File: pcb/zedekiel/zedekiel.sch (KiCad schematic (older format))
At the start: 150 parts, among them K1 KEYSW, K10 KEYSW, K11 KEYSW, K12 KEYSW, K13 KEYSW, K14 KEYSW, K15 KEYSW, K16 KEYSW, K17 KEYSW, K18 KEYSW, K19 KEYSW, K2 KEYSW, K20 KEYSW, K21 KEYSW, K22 KEYSW, K23 KEYSW, K24 KEYSW, K25 KEYSW, K26 KEYSW, K27 KEYSW, K28 KEYSW, K29 KEYSW, K3 KEYSW, K30 KEYSW, K31 KEYSW, K32 KEYSW, K33 KEYSW, K34 KEYSW, K35 KEYSW, K36 KEYSW, K37 KEYSW, K38 KEYSW, K39 KEYSW, K4 KEYSW, K40 KEYSW, K41 KEYSW, K42 KEYSW, K43 KEYSW, K44 KEYSW, K45 KEYSW, K46 KEYSW, K47 KEYSW, K48 KEYSW, K49 KEYSW, K5 KEYSW, K50 KEYSW, K51 KEYSW, K52 KEYSW, K53 KEYSW, K54 KEYSW, K55 KEYSW, K56 KEYSW, K57 KEYSW, K58 KEYSW, K59 KEYSW, K6 KEYSW, K60 KEYSW, K61 KEYSW, K62 KEYSW, K63 KEYSW, K64 KEYSW, K65 KEYSW, K66 KEYSW, K7 KEYSW, K8 KEYSW, K9 KEYSW, SW1 SW_PUSH, U1 ATmega16U4-AU_(modified), X1 16MHz

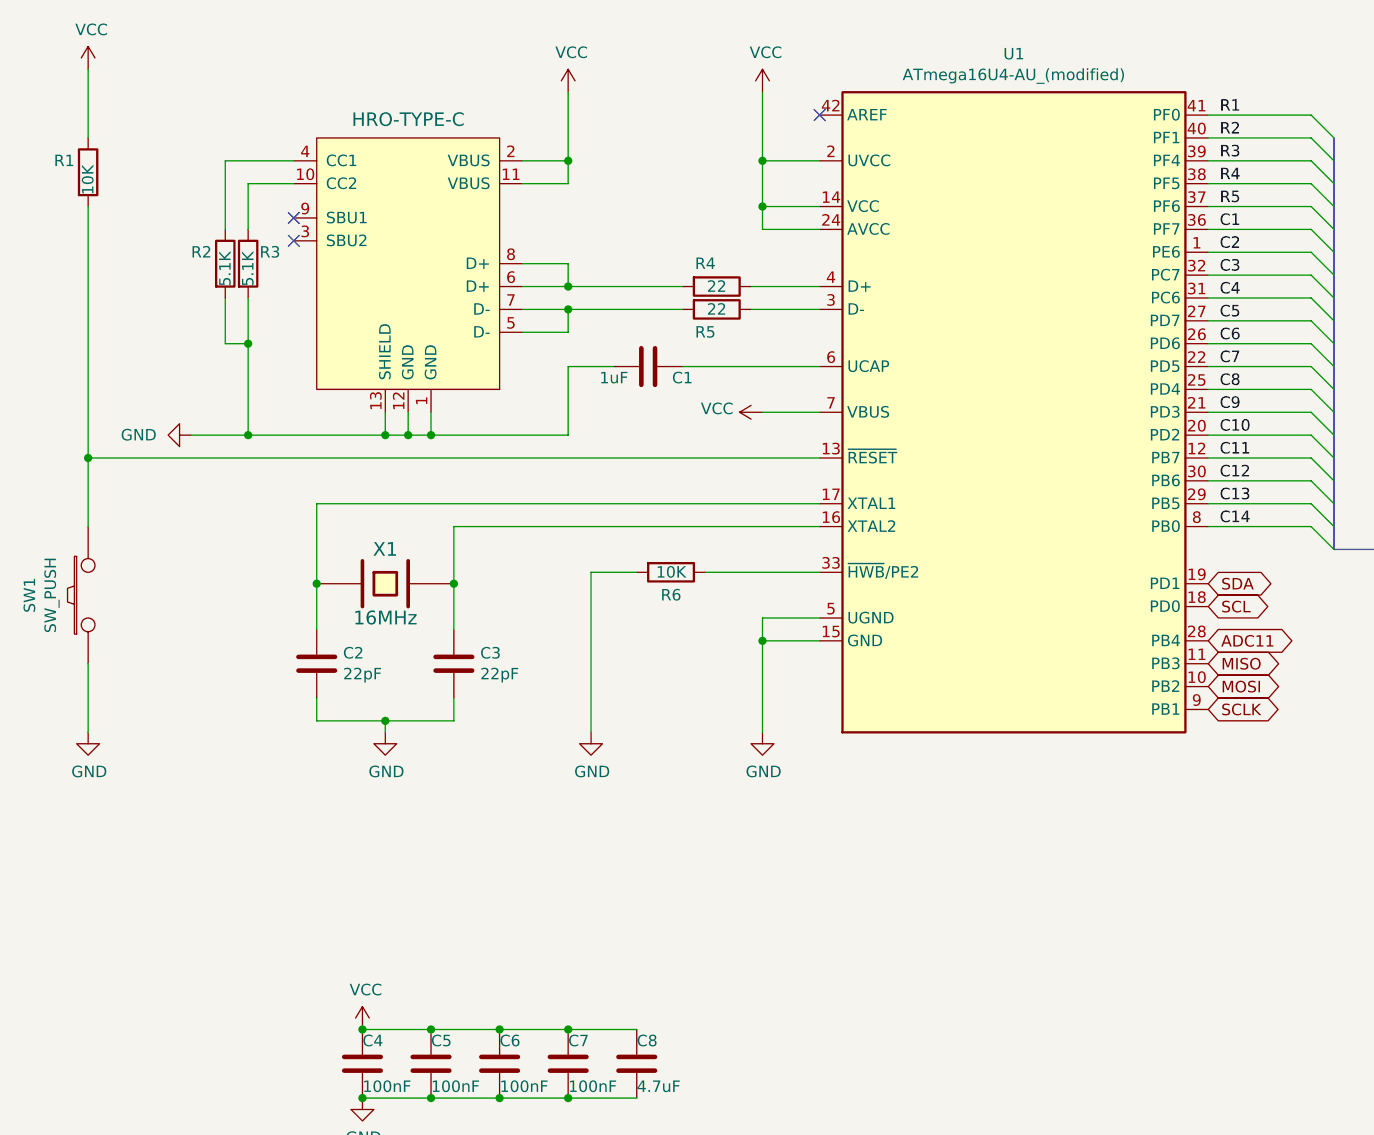
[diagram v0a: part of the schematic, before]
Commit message: Pads
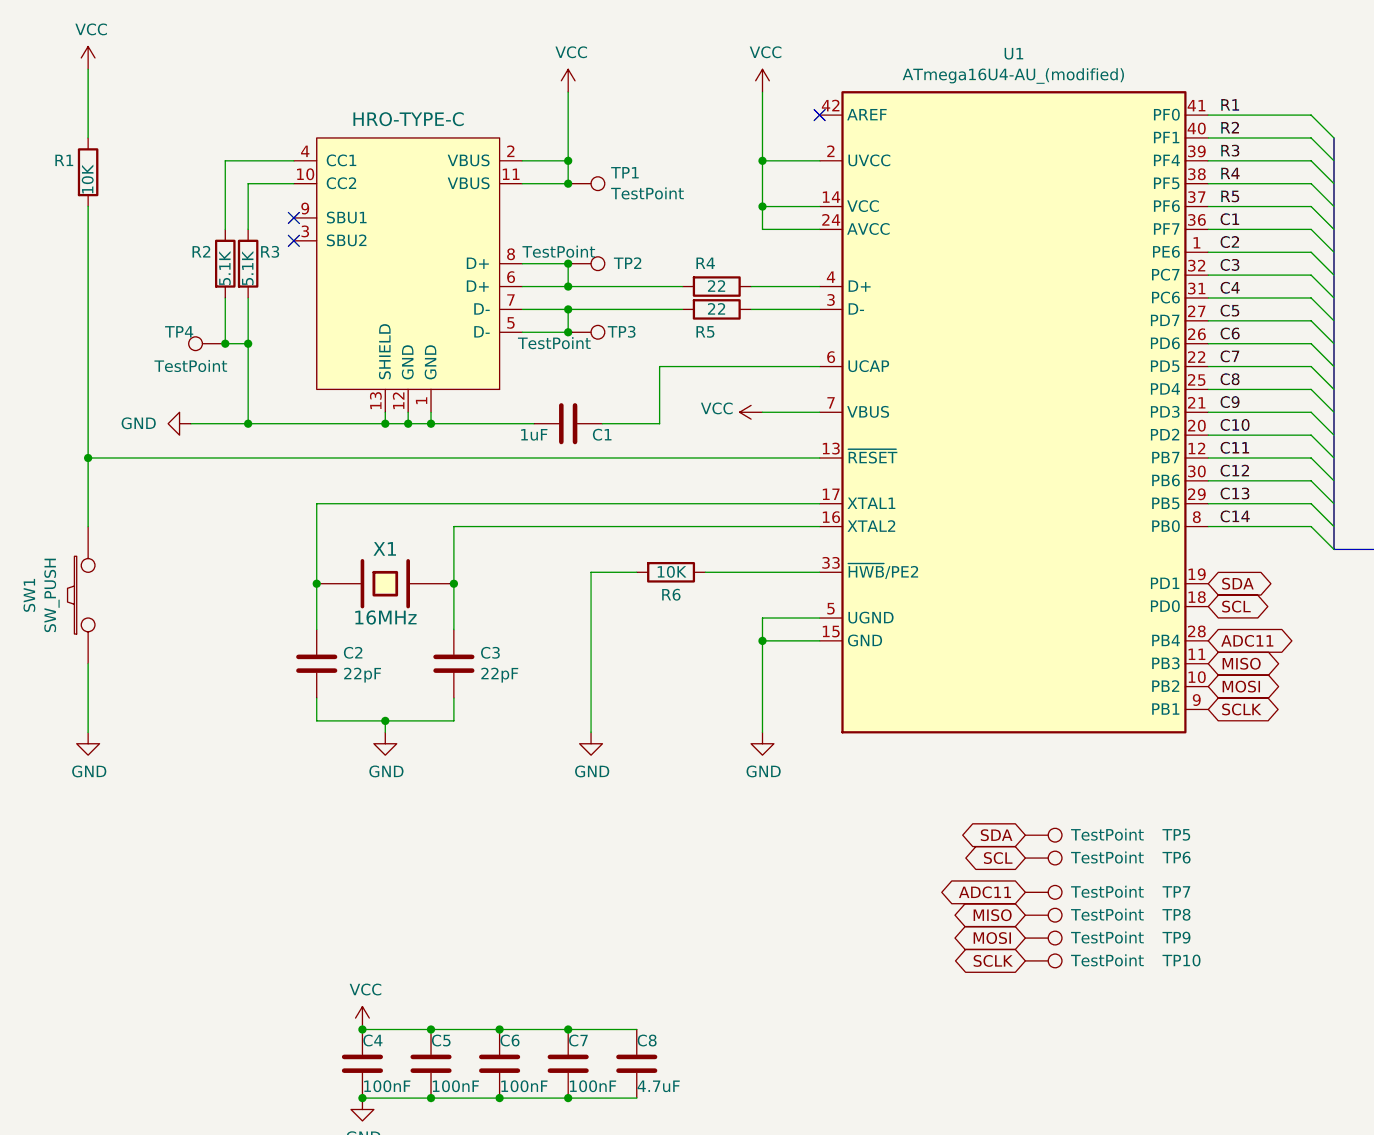
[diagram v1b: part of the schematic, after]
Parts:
- added TP1, TP10, TP2, TP3, TP4, TP5, TP6, TP7, TP8, TP9: TestPoint, custom:single-pad, symbol Connector:TestPoint
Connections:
- net ADC11: now also TP7.1
- net GND: now also TP4.1
- net MISO: now also TP8.1
- net MOSI: now also TP9.1
- net SCL: now also TP6.1
- net SCLK: now also TP10.1
- net SDA: now also TP5.1
- net VCC: now also TP1.1
- net at R4.2, USB1.6 (D+), USB1.8 (D+): now also TP2.1
- net at R5.2, USB1.5 (D-), USB1.7 (D-): now also TP3.1
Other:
- moved on the sheet: C1
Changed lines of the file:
@@
 	4550 2650 4300 2650
-$Comp
-L Device:C C1
-U 1 1 5EE5A2F4
-P 3800 2450
-F 0 "C1" V 3850 2600 50  0000 C CNN
-F 1 "1uF" V 3850 2300 50  0000 C CNN
-F 2 "Capacitors_SMD:C_0603" H 3838 2300 50  0001 C CNN
-F 3 "~" H 3800 2450 50  0001 C CNN
-	1    3800 2450
-	0    1    1    0
-$EndComp
-Wire Wire Line
-	3950 2450 4550 2450
 $Comp
 L keyboard_parts:SW_PUSH SW1
@@
 L power:GND #PWR04
 U 1 1 5EE60D7B
-P 1800 2750
-F 0 "#PWR04" H 1800 2500 50  0001 C CNN
-F 1 "GND" V 1800 2600 50  0000 R CNN
-F 2 "" H 1800 2750 50  0001 C CNN
-F 3 "" H 1800 2750 50  0001 C CNN
-	1    1800 2750
+P 1800 2700
+F 0 "#PWR04" H 1800 2450 50  0001 C CNN
+F 1 "GND" V 1800 2550 50  0000 R CNN
+F 2 "" H 1800 2700 50  0001 C CNN
+F 3 "" H 1800 2700 50  0001 C CNN
+	1    1800 2700
 	0    1    1    0
 $EndComp
@@
 Wire Wire Line
 	3450 2200 3450 2300
-Wire Wire Line
-	3450 2300 3250 2300
-Wire Wire Line
-	3450 2200 3950 2200
 Connection ~ 3450 2200
 Wire Wire Line
@@
 Connection ~ 3450 2100
 Wire Wire Line
-	3950 2100 3450 2100
-Wire Wire Line
 	3450 2100 3250 2100
 Wire Wire Line
@@
 Connection ~ 3450 1550
 Wire Wire Line
-	2050 2350 2050 2750
-Wire Wire Line
-	3650 2450 3450 2450
-Wire Wire Line
-	3450 2450 3450 2750
-Wire Wire Line
-	3450 2750 2850 2750
-Wire Wire Line
-	2850 2650 2850 2750
-Connection ~ 2850 2750
-Wire Wire Line
-	2850 2750 2750 2750
-Wire Wire Line
-	2750 2650 2750 2750
-Connection ~ 2750 2750
-Wire Wire Line
-	2750 2750 2650 2750
-Wire Wire Line
-	2650 2650 2650 2750
-Connection ~ 2650 2750
-Wire Wire Line
-	2650 2750 2050 2750
-Connection ~ 2050 2750
-Wire Wire Line
-	2050 2750 1800 2750
+	2050 2350 2050 2700
+Wire Wire Line
+	2850 2650 2850 2700
+Connection ~ 2850 2700
+Wire Wire Line
+	2850 2700 2750 2700
+Wire Wire Line
+	2750 2650 2750 2700
+Connection ~ 2750 2700
+Wire Wire Line
+	2750 2700 2650 2700
+Wire Wire Line
+	2650 2650 2650 2700
+Connection ~ 2650 2700
+Wire Wire Line
+	2650 2700 2050 2700
+Connection ~ 2050 2700
+Wire Wire Line
+	2050 2700 1800 2700
 Wire Wire Line
 	1350 1750 1350 2850
 Wire Wire Line
 	4550 2850 1350 2850
+Connection ~ 1350 2850
+Wire Wire Line
+	1350 2850 1350 3150
+$Comp
+L Connector:TestPoint TP2
+U 1 1 5F0D5D9F
+P 3450 2000
+F 0 "TP2" V 3450 2200 50  0000 L CNN
+F 1 "TestPoint" V 3400 1800 50  0000 L CNN
+F 2 "custom:single-pad" H 3650 2000 50  0001 C CNN
+F 3 "~" H 3650 2000 50  0001 C CNN
+	1    3450 2000
+	0    1    1    0
+$EndComp
+$Comp
+L Connector:TestPoint TP3
+U 1 1 5F0E41D9
+P 3450 2300
+F 0 "TP3" V 3450 2600 50  0000 R CNN
+F 1 "TestPoint" V 3500 2400 50  0000 R CNN
+F 2 "custom:single-pad" H 3650 2300 50  0001 C CNN
+F 3 "~" H 3650 2300 50  0001 C CNN
+	1    3450 2300
+	0    1    1    0
+$EndComp
+Connection ~ 3450 2000
+Wire Wire Line
+	3450 2100 3950 2100
+Wire Wire Line
+	3450 2200 3950 2200
+Connection ~ 3450 2300
+Wire Wire Line
+	3250 2300 3450 2300
+$Comp
+L Connector:TestPoint TP1
+U 1 1 5F0FDFC9
+P 3450 1650
+F 0 "TP1" V 3404 1838 50  0000 L CNN
+F 1 "TestPoint" V 3495 1838 50  0000 L CNN
+F 2 "custom:single-pad" H 3650 1650 50  0001 C CNN
+F 3 "~" H 3650 1650 50  0001 C CNN
+	1    3450 1650
+	0    1    1    0
+$EndComp
+Connection ~ 3450 1650
+$Comp
+L Connector:TestPoint TP4
+U 1 1 5F100506
+P 1950 2350
+F 0 "TP4" V 2000 2550 50  0000 C CNN
+F 1 "TestPoint" V 1850 2500 50  0000 C CNN
+F 2 "custom:single-pad" H 2150 2350 50  0001 C CNN
+F 3 "~" H 2150 2350 50  0001 C CNN
+	1    1950 2350
+	0    -1   -1   0
+$EndComp
+Connection ~ 1950 2350
+Wire Wire Line
+	3300 2700 2850 2700
+$Comp
+L Device:C C1
+U 1 1 5EE5A2F4
+P 3450 2700
+F 0 "C1" V 3500 2850 50  0000 C CNN
+F 1 "1uF" V 3500 2550 50  0000 C CNN
+F 2 "Capacitors_SMD:C_0603" H 3488 2550 50  0001 C CNN
+F 3 "~" H 3450 2700 50  0001 C CNN
+	1    3450 2700
+	0    1    1    0
+$EndComp
+Wire Wire Line
+	3600 2700 3850 2700
+Wire Wire Line
+	3850 2700 3850 2450
+Wire Wire Line
+	3850 2450 4550 2450
+Text GLabel 5450 4500 0    50   BiDi ~ 0
+SDA
+Text GLabel 5450 4600 0    50   BiDi ~ 0
+SCL
+Text GLabel 5450 4750 0    50   BiDi ~ 0
+ADC11
+Text GLabel 5450 4850 0    50   BiDi ~ 0
+MISO
+Text GLabel 5450 4950 0    50   BiDi ~ 0
+MOSI
+Text GLabel 5450 5050 0    50   BiDi ~ 0
+SCLK
+$Comp
+L Connector:TestPoint TP5
+U 1 1 5F2116B9
+P 5450 4500
+F 0 "TP5" V 5450 5100 50  0000 L CNN
+F 1 "TestPoint" V 5450 4700 50  0000 L CNN
+F 2 "custom:single-pad" H 5650 4500 50  0001 C CNN
+F 3 "~" H 5650 4500 50  0001 C CNN
+	1    5450 4500
+	0    1    1    0
+$EndComp
+$Comp
+L Connector:TestPoint TP6
+U 1 1 5F212DC2
+P 5450 4600
+F 0 "TP6" V 5450 5200 50  0000 L CNN
+F 1 "TestPoint" V 5450 4800 50  0000 L CNN
+F 2 "custom:single-pad" H 5650 4600 50  0001 C CNN
+F 3 "~" H 5650 4600 50  0001 C CNN
+	1    5450 4600
+	0    1    1    0
+$EndComp
+$Comp
+L Connector:TestPoint TP7
+U 1 1 5F21FF89
+P 5450 4750
+F 0 "TP7" V 5450 5350 50  0000 L CNN
+F 1 "TestPoint" V 5450 4950 50  0000 L CNN
+F 2 "custom:single-pad" H 5650 4750 50  0001 C CNN
+F 3 "~" H 5650 4750 50  0001 C CNN
+	1    5450 4750
+	0    1    1    0
+$EndComp
+$Comp
+L Connector:TestPoint TP8
+U 1 1 5F22D0CC
+P 5450 4850
+F 0 "TP8" V 5450 5450 50  0000 L CNN
+F 1 "TestPoint" V 5450 5050 50  0000 L CNN
+F 2 "custom:single-pad" H 5650 4850 50  0001 C CNN
+F 3 "~" H 5650 4850 50  0001 C CNN
+	1    5450 4850
+	0    1    1    0
+$EndComp
+$Comp
+L Connector:TestPoint TP9
+U 1 1 5F23B9EB
+P 5450 4950
+F 0 "TP9" V 5450 5550 50  0000 L CNN
+F 1 "TestPoint" V 5450 5150 50  0000 L CNN
+F 2 "custom:single-pad" H 5650 4950 50  0001 C CNN
+F 3 "~" H 5650 4950 50  0001 C CNN
+	1    5450 4950
+	0    1    1    0
+$EndComp
+$Comp
+L Connector:TestPoint TP10
+U 1 1 5F248B64
+P 5450 5050
+F 0 "TP10" V 5450 5650 50  0000 L CNN
+F 1 "TestPoint" V 5450 5250 50  0000 L CNN
+F 2 "custom:single-pad" H 5650 5050 50  0001 C CNN
+F 3 "~" H 5650 5050 50  0001 C CNN
+	1    5450 5050
+	0    1    1    0
+$EndComp
 Wire Bus Line
 	7300 1200 7300 3250
@@
 Wire Bus Line
 	6800 1450 6800 3250
-Connection ~ 1350 2850
-Wire Wire Line
-	1350 2850 1350 3150
 $EndSCHEMATC
